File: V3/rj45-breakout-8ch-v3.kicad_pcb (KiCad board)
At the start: 2 copper layers, 93 x 67.8 mm, 13 parts, among them J1 Jack RJ45, J10 Conn_01x06, J11 Conn_01x06, J12 Conn_01x06, J13 Conn_01x06, J2 Jack RJ45, J3 Jack RJ45, J4 Jack RJ45, J5 Jack RJ45, J6 Jack RJ45, J7 Jack RJ45, J8 Jack RJ45, J9 Conn_01x02

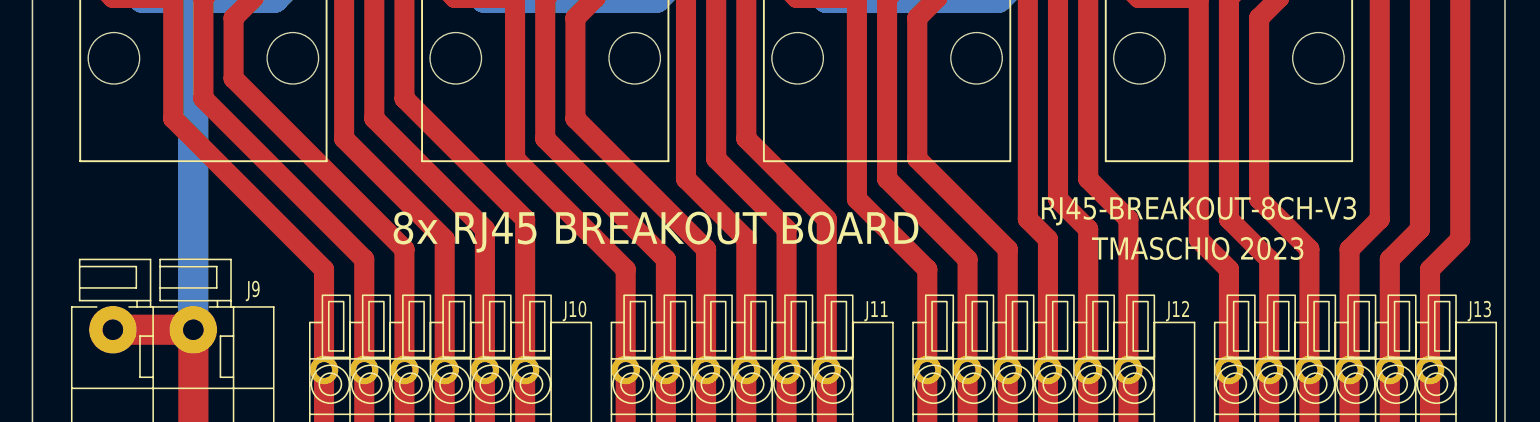
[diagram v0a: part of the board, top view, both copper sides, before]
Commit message: Layout tweakings
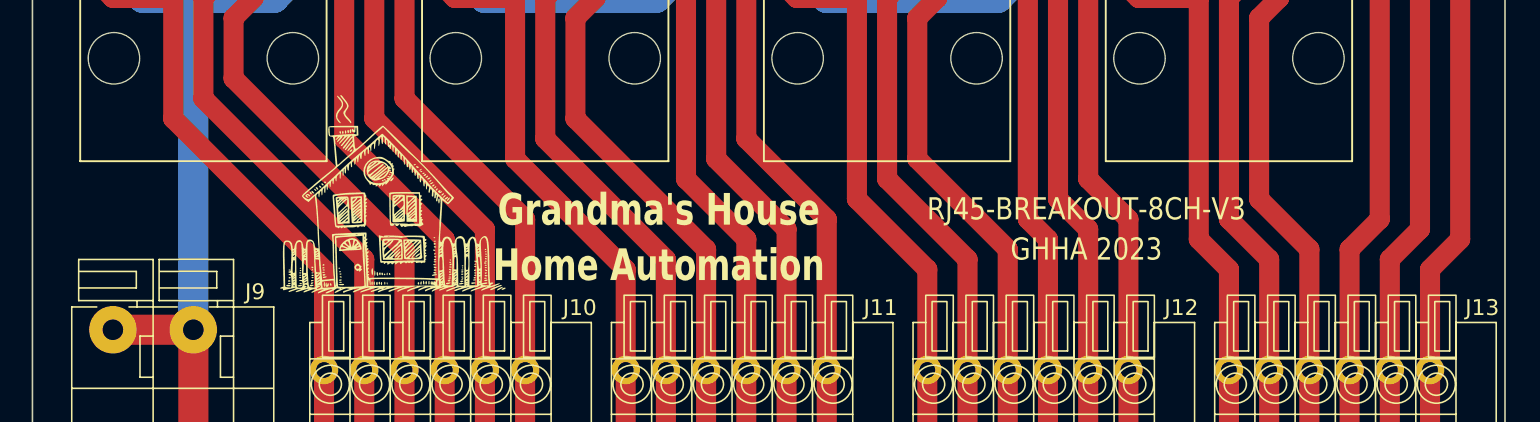
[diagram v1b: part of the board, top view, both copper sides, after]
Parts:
- added ?: , Tales:Grandmas_medium, F.Cu at (114.1, 103.8)
- J10: value Conn_01x06 -> SWITCHES1; footprint Tales:TerminalBlock_Phoenix_FFKDSA1-V-2.54-6_1x06_P2.54mm_Vertical -> Tales:TerminalBlock_DB141V-2.54-6P_1x06_P2.54mm_Vertical
- J11: value Conn_01x06 -> SWITCHES2; footprint Tales:TerminalBlock_Phoenix_FFKDSA1-V-2.54-6_1x06_P2.54mm_Vertical -> Tales:TerminalBlock_DB141V-2.54-6P_1x06_P2.54mm_Vertical
- J12: value Conn_01x06 -> SWITCHES3; footprint Tales:TerminalBlock_Phoenix_FFKDSA1-V-2.54-6_1x06_P2.54mm_Vertical -> Tales:TerminalBlock_DB141V-2.54-6P_1x06_P2.54mm_Vertical
- J13: value Conn_01x06 -> SWITCHES4; footprint Tales:TerminalBlock_Phoenix_FFKDSA1-V-2.54-6_1x06_P2.54mm_Vertical -> Tales:TerminalBlock_DB141V-2.54-6P_1x06_P2.54mm_Vertical
- J9: value Conn_01x02 -> 24V; footprint Tales:TerminalBlock_Phoenix_FFKDSA-V1-5.08-2_1x02_P5.08mm_Vertical -> Tales:TerminalBlock_DB142V-2-5.08_1x02_P5.08mm_Vertical
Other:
- board text added: "GHHA 2023"
- board text added: "Grandma's House"
- board text added: "Home Automation"
- board text removed: "8x RJ45 BREAKOUT BOARD"
- board text removed: "TMASCHIO 2023"
